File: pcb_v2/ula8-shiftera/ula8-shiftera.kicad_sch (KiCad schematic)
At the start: 17 parts, among them J1 ula8a, U1 74LS244, U2 74LS244, U3 74LS157, U4 74LS157

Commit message: deslocando alimentação para as estremidades do conector; carry out em três estados (ativo apenas quando select)
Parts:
- added C5, C6, C7: 100nF, Capacitor_THT:C_Disc_D5.1mm_W3.2mm_P5.00mm, symbol Device:C
- added U5: 74LS125, Package_DIP:DIP-14_W7.62mm, symbol 74xx:74LS125
- added U6, U7, U8: 74LS244, Package_DIP:DIP-20_W7.62mm, symbol 74xx:74LS244
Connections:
- net +5V: now also C5.2, C6.2, C7.2, U5.1, U5.10, U5.14 (VCC), U5.2, U5.4, U5.5, U5.9, U6.20 (VCC), U7.20 (VCC)
- net GND: now also C5.1, C6.1, C7.1, U5.7 (GND), U6.10 (GND), U7.10 (GND)
- net carry_out: now also U5.11; no longer U4.4 (Za)
- net lower_bus0: now also U6.4 (I1a)
- net lower_bus1: now also U6.6 (I2a), U7.2 (I0a)
- net lower_bus2: now also U6.8 (I3a), U7.4 (I1a)
- net lower_bus3: now also U6.11 (I0b), U7.6 (I2a)
- net lower_bus4: now also U6.13 (I1b), U7.8 (I3a)
- net lower_bus5: now also U6.15 (I2b), U7.11 (I0b)
- net lower_bus6: now also U6.17 (I3b), U7.13 (I1b)
- net lower_bus7: now also U7.15 (I2b)
- net ula_bus0: now also U6.18 (O0a), U7.18 (O0a)
- net ula_bus1: now also U6.16 (O1a), U7.16 (O1a)
- net ula_bus2: now also U6.14 (O2a), U7.14 (O2a)
- net ula_bus3: now also U6.12 (O3a), U7.12 (O3a)
- net ula_bus4: now also U6.9 (O0b), U7.9 (O0b)
- net ula_bus5: now also U6.7 (O1b), U7.7 (O1b)
- net ula_bus6: now also U6.5 (O2b), U7.5 (O2b)
- net ula_bus7: now also U6.3 (O3b), U7.3 (O3b)
- net ~{select}: now also U5.13
- net ~{shift_left}: now also U6.1 (OEa), U6.19 (OEb)
- net ~{shift_right}: now also U7.1 (OEa), U7.19 (OEb)
- net option_rigth renamed option_right
- new net: U4.4 (Za), U5.12
- new net new_bit_0: U6.2 (I0a), U7.17 (I3b)
- no-connect marks 22 -> 25
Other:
- moved on the sheet: C1, C2, C3, C4, U1, U2, U3, U4

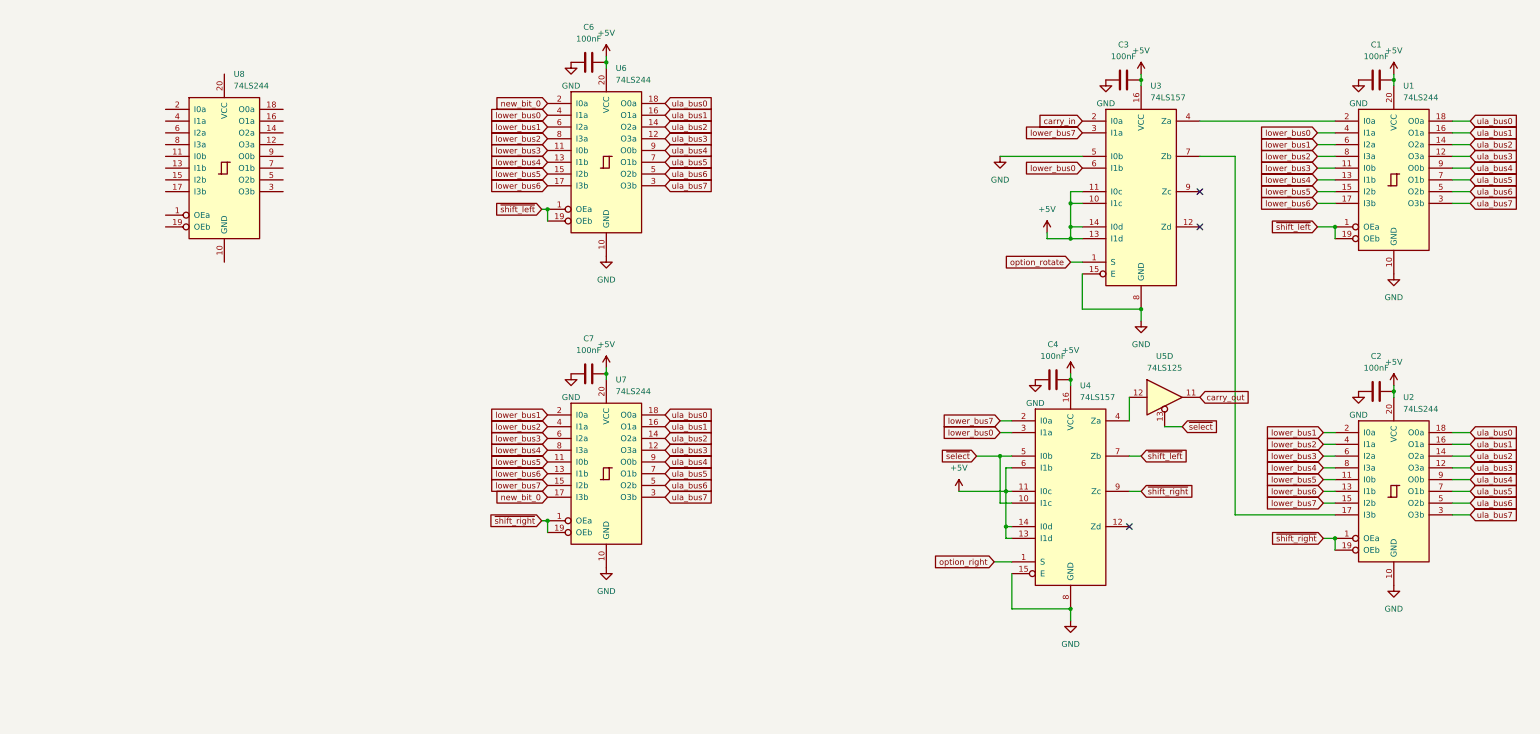
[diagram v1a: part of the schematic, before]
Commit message: faltava salvar
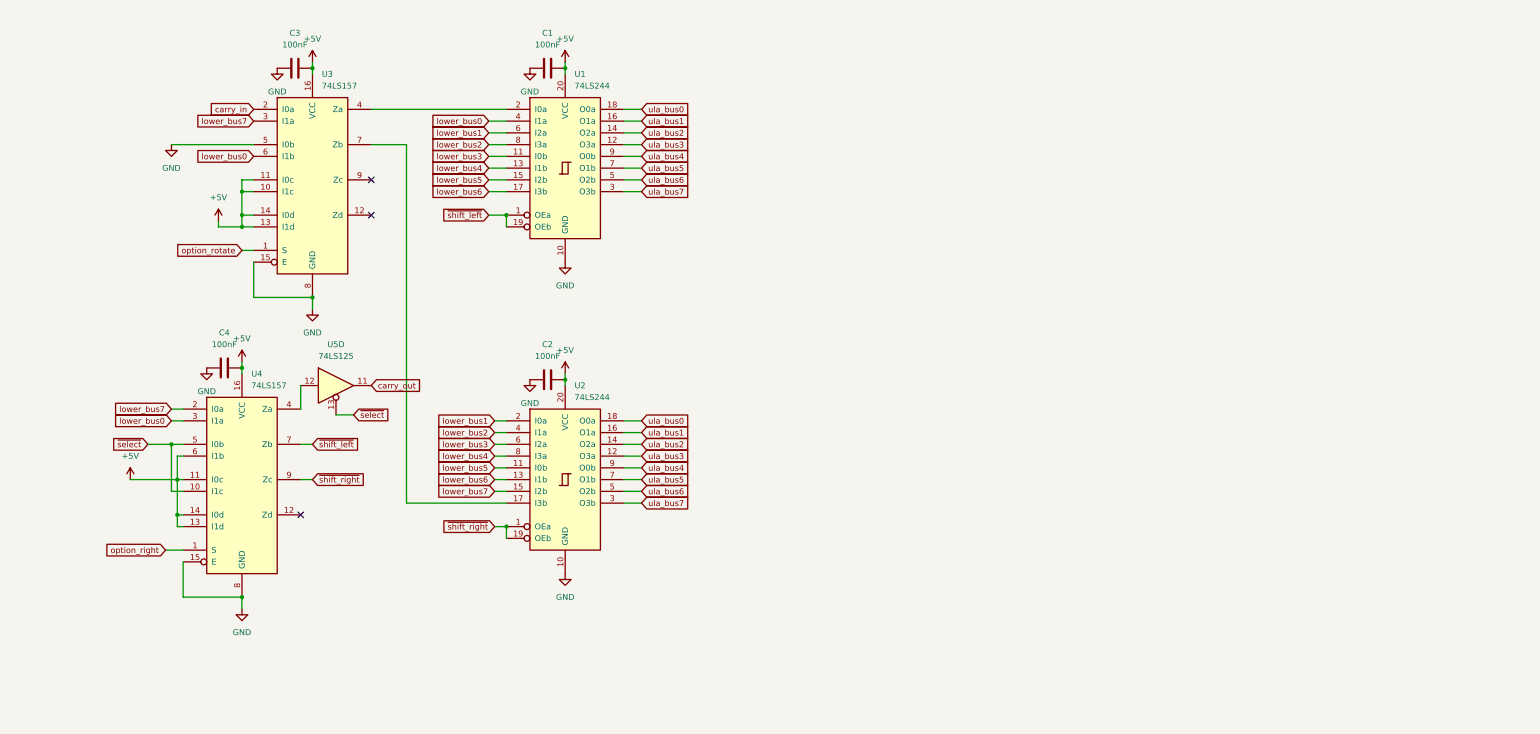
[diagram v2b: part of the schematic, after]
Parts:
- removed C6, C7: 100nF, Capacitor_THT:C_Disc_D5.1mm_W3.2mm_P5.00mm, symbol Device:C
- removed U6, U7, U8: 74LS244, Package_DIP:DIP-20_W7.62mm, symbol 74xx:74LS244
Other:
- moved on the sheet: C1, C2, C3, C4, U1, U2, U3, U4, U5D
